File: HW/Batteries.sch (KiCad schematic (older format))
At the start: 18 parts

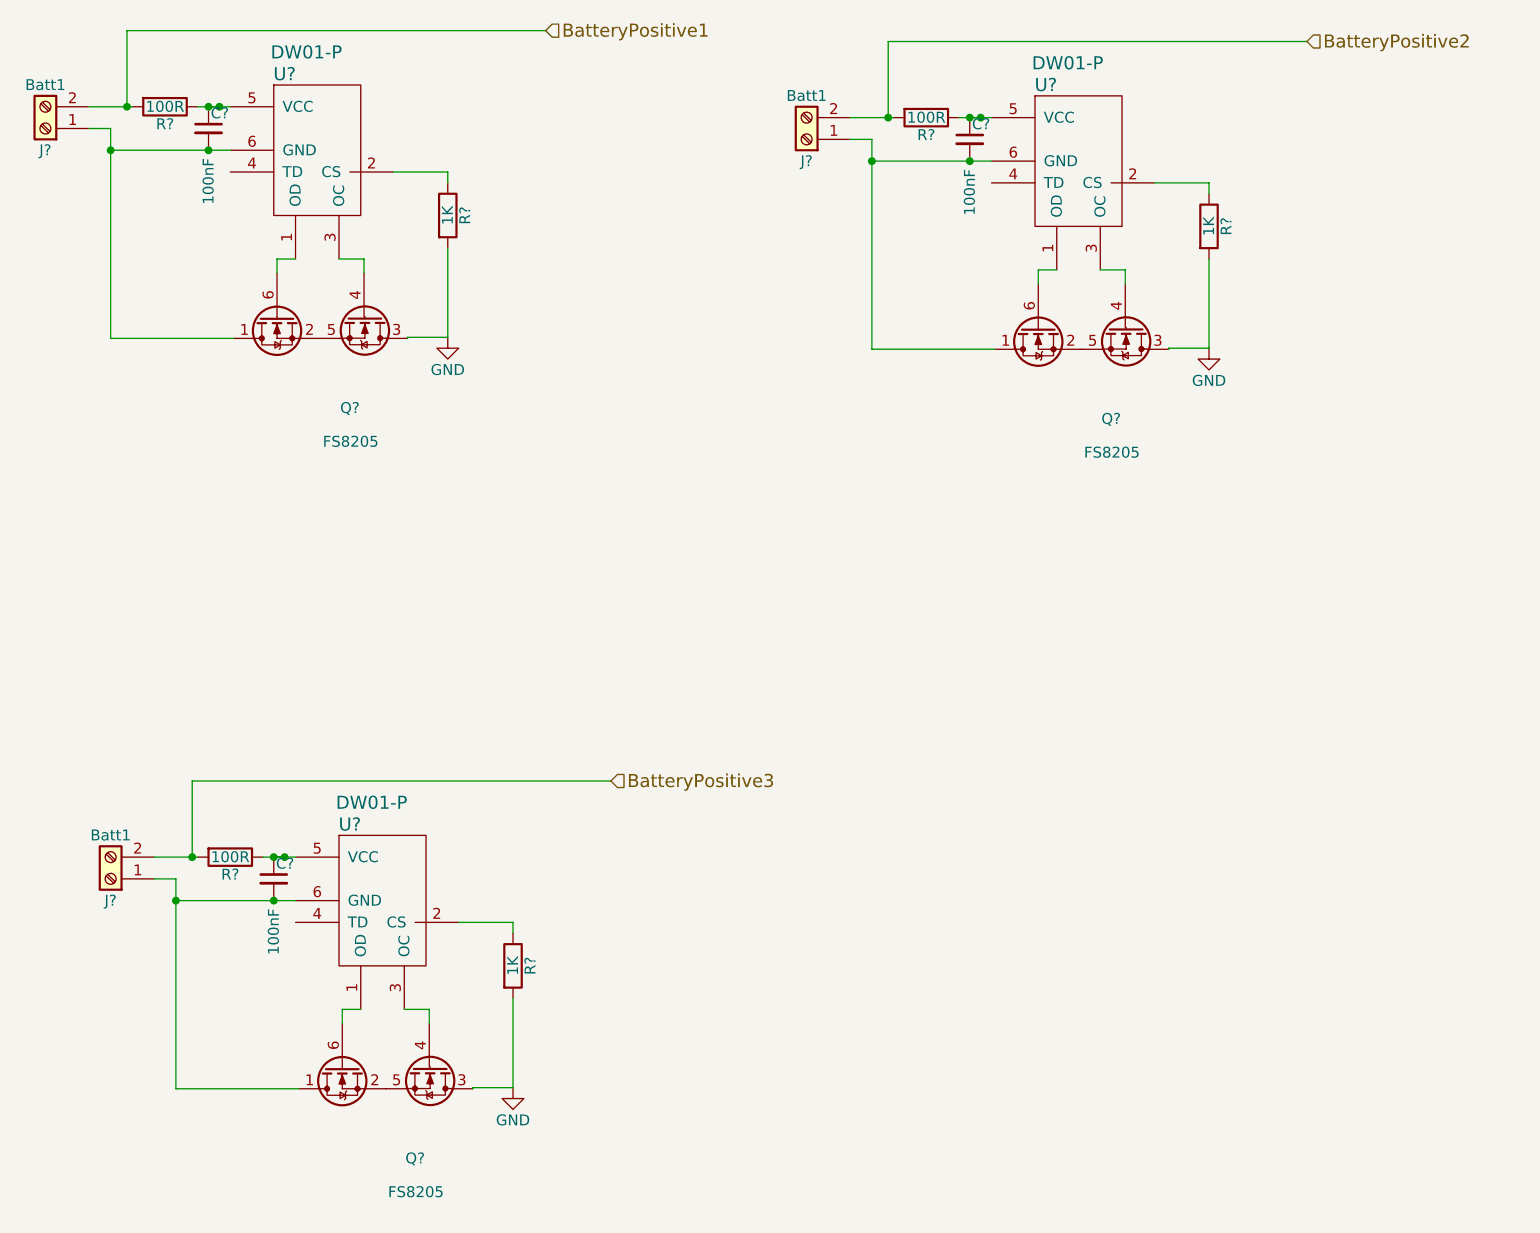
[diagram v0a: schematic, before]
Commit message: Add files via upload
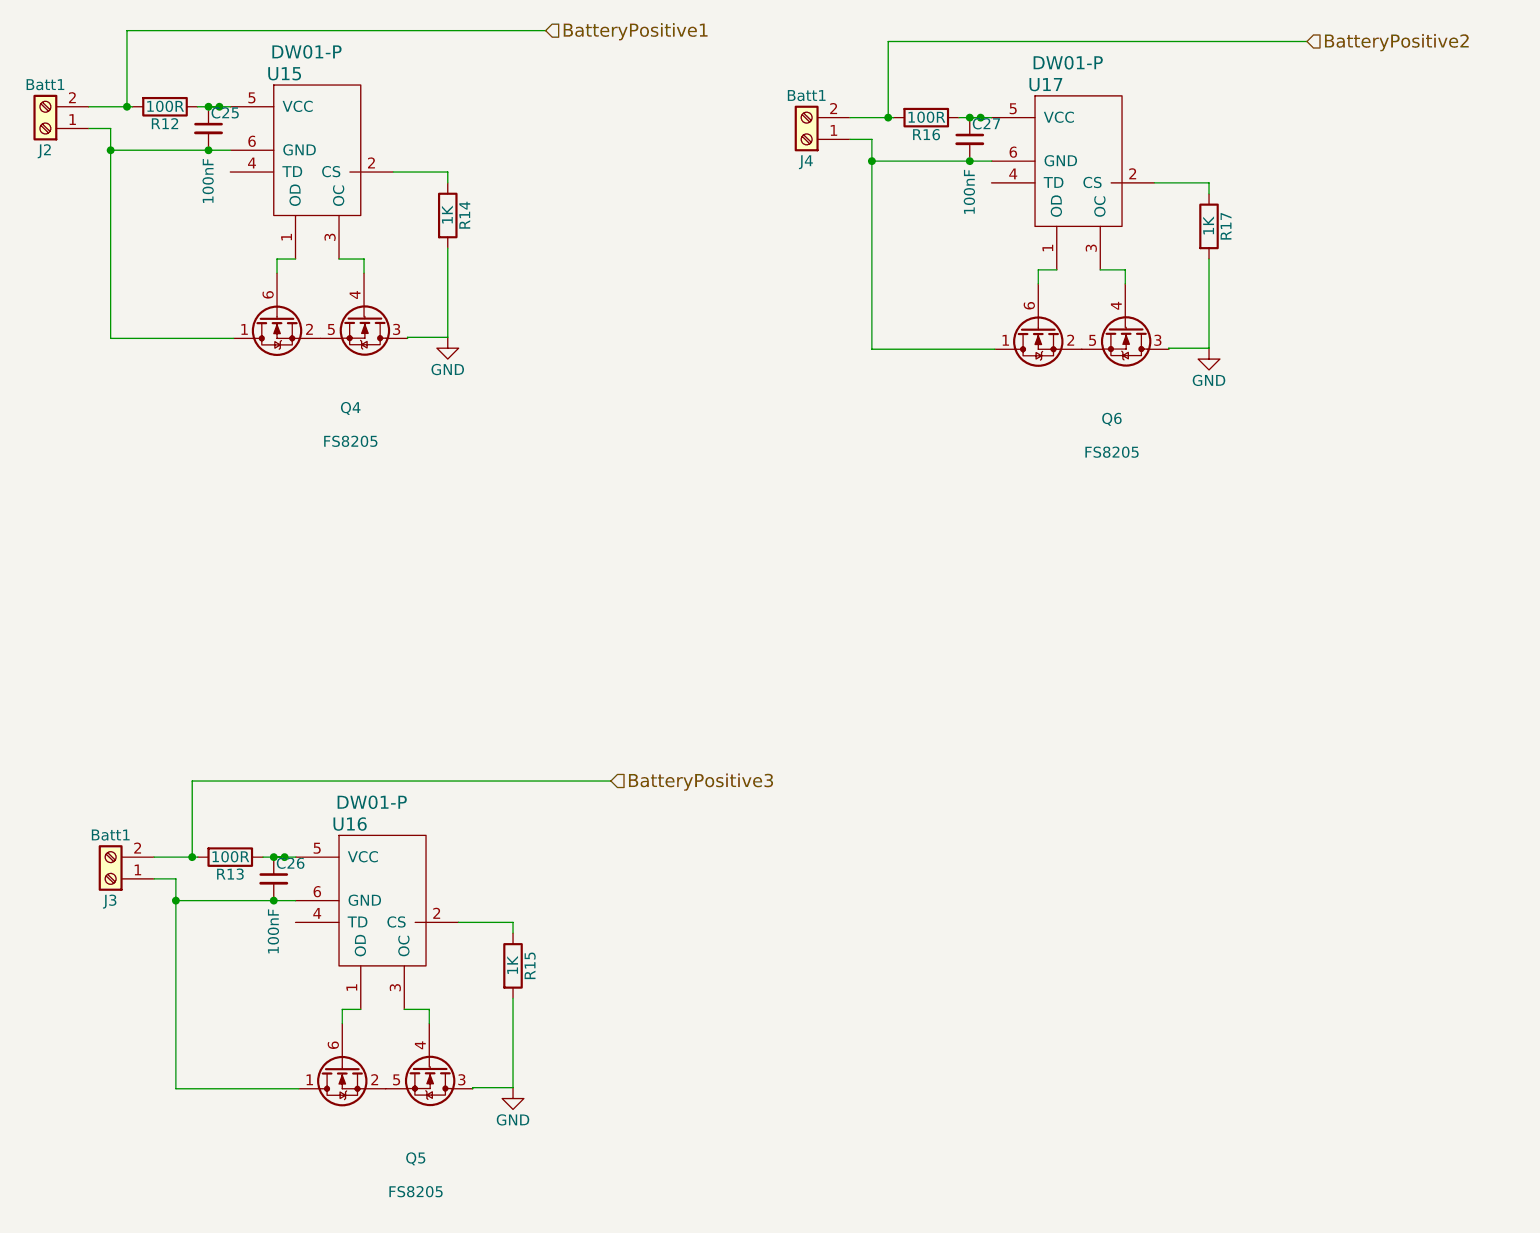
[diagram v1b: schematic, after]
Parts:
- C25, C26, C27: renamed from C?; footprint (none) -> Capacitors_SMD:C_0805_HandSoldering
- J2, J3, J4: renamed from J?; footprint (none) -> Connectors_Terminal_Blocks:TerminalBlock_bornier-2_P5.08mm
- R12, R13, R14, R15, R16, R17: renamed from R?; footprint (none) -> Resistors_SMD:R_0805_HandSoldering
- gave numbers to parts that had none: 6
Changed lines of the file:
@@
 LIBS:Peters
 LIBS:WS2812B
-LIBS:pro-mini-cache
+LIBS:discharger-cache
 EELAYER 25 0
 EELAYER END
@@
 BatteryPositive3
 $Comp
-L R R?
+L R R16
 U 1 1 5A983102
 P 5350 1600
-F 0 "R?" V 5430 1600 50  0000 C CNN
+F 0 "R16" V 5430 1600 50  0000 C CNN
 F 1 "100R" V 5350 1600 50  0000 C CNN
-F 2 "" V 5280 1600 50  0001 C CNN
+F 2 "Resistors_SMD:R_0805_HandSoldering" V 5280 1600 50  0001 C CNN
 F 3 "" H 5350 1600 50  0001 C CNN
 	1    5350 1600
@@
 $EndComp
 $Comp
-L C_Small C?
+L C_Small C27
 U 1 1 5A983108
 P 5550 1700
-F 0 "C?" H 5560 1770 50  0000 L CNN
+F 0 "C27" H 5560 1770 50  0000 L CNN
 F 1 "100nF" V 5550 1350 50  0000 L CNN
-F 2 "" H 5550 1700 50  0001 C CNN
+F 2 "Capacitors_SMD:C_0805_HandSoldering" H 5550 1700 50  0001 C CNN
 F 3 "" H 5550 1700 50  0001 C CNN
 	1    5550 1700
@@
 $EndComp
 $Comp
-L R R?
+L R R17
 U 1 1 5A98310E
 P 6650 2100
-F 0 "R?" V 6730 2100 50  0000 C CNN
+F 0 "R17" V 6730 2100 50  0000 C CNN
 F 1 "1K" V 6650 2100 50  0000 C CNN
-F 2 "" V 6580 2100 50  0001 C CNN
+F 2 "Resistors_SMD:R_0805_HandSoldering" V 6580 2100 50  0001 C CNN
 F 3 "" H 6650 2100 50  0001 C CNN
 	1    6650 2100
@@
 $EndComp
 $Comp
-L FS8205 Q?
+L FS8205 Q6
 U 1 1 5A983114
 P 6065 2665
-F 0 "Q?" H 6155 2345 50  0000 L CNN
+F 0 "Q6" H 6155 2345 50  0000 L CNN
 F 1 "FS8205" H 6075 2190 50  0000 L CNN
 F 2 "TO_SOT_Packages_SMD:SOT-23-6_Handsoldering" H 5125 2065 50  0001 L CIN
@@
 $EndComp
 $Comp
-L Screw_Terminal_01x02 J?
+L Screw_Terminal_01x02 J4
 U 1 1 5A98311A
 P 4800 1700
-F 0 "J?" H 4800 1800 50  0000 C CNN
+F 0 "J4" H 4800 1800 50  0000 C CNN
 F 1 "Batt1" H 4800 1500 50  0000 C CNN
-F 2 "" H 4800 1700 50  0001 C CNN
+F 2 "Connectors_Terminal_Blocks:TerminalBlock_bornier-2_P5.08mm" H 4800 1700 50  0001 C CNN
 F 3 "" H 4800 1700 50  0001 C CNN
 	1    4800 1700
@@
 $EndComp
 $Comp
-L GND #PWR?
+L GND #PWR92
 U 1 1 5A983120
 P 6650 2660
-F 0 "#PWR?" H 6650 2410 50  0001 C CNN
+F 0 "#PWR92" H 6650 2410 50  0001 C CNN
 F 1 "GND" H 6650 2510 50  0000 C CNN
 F 2 "" H 6650 2660 50  0001 C CNN
@@
 Connection ~ 5175 1600
 $Comp
-L DW01-P U?
+L DW01-P U17
 U 1 1 5A983132
 P 6000 1700
-F 0 "U?" H 5900 1950 60  0000 C CNN
+F 0 "U17" H 5900 1950 60  0000 C CNN
 F 1 "DW01-P" H 6000 2050 60  0000 C CNN
 F 2 "TO_SOT_Packages_SMD:SOT-23-6_Handsoldering" H 5750 2150 60  0001 C CNN
@@
 	5100 1800 5650 1800
 $Comp
-L R R?
+L R R12
 U 1 1 5A983DEE
 P 1850 1550
-F 0 "R?" V 1930 1550 50  0000 C CNN
+F 0 "R12" V 1930 1550 50  0000 C CNN
 F 1 "100R" V 1850 1550 50  0000 C CNN
-F 2 "" V 1780 1550 50  0001 C CNN
+F 2 "Resistors_SMD:R_0805_HandSoldering" V 1780 1550 50  0001 C CNN
 F 3 "" H 1850 1550 50  0001 C CNN
 	1    1850 1550
@@
 $EndComp
 $Comp
-L C_Small C?
+L C_Small C25
 U 1 1 5A983DF4
 P 2050 1650
-F 0 "C?" H 2060 1720 50  0000 L CNN
+F 0 "C25" H 2060 1720 50  0000 L CNN
 F 1 "100nF" V 2050 1300 50  0000 L CNN
-F 2 "" H 2050 1650 50  0001 C CNN
+F 2 "Capacitors_SMD:C_0805_HandSoldering" H 2050 1650 50  0001 C CNN
 F 3 "" H 2050 1650 50  0001 C CNN
 	1    2050 1650
@@
 $EndComp
 $Comp
-L R R?
+L R R14
 U 1 1 5A983DFA
 P 3150 2050
-F 0 "R?" V 3230 2050 50  0000 C CNN
+F 0 "R14" V 3230 2050 50  0000 C CNN
 F 1 "1K" V 3150 2050 50  0000 C CNN
-F 2 "" V 3080 2050 50  0001 C CNN
+F 2 "Resistors_SMD:R_0805_HandSoldering" V 3080 2050 50  0001 C CNN
 F 3 "" H 3150 2050 50  0001 C CNN
 	1    3150 2050
@@
 $EndComp
 $Comp
-L FS8205 Q?
+L FS8205 Q4
 U 1 1 5A983E00
 P 2565 2615
-F 0 "Q?" H 2655 2295 50  0000 L CNN
+F 0 "Q4" H 2655 2295 50  0000 L CNN
 F 1 "FS8205" H 2575 2140 50  0000 L CNN
 F 2 "TO_SOT_Packages_SMD:SOT-23-6_Handsoldering" H 1625 2015 50  0001 L CIN
@@
 $EndComp
 $Comp
-L Screw_Terminal_01x02 J?
+L Screw_Terminal_01x02 J2
 U 1 1 5A983E06
 P 1300 1650
-F 0 "J?" H 1300 1750 50  0000 C CNN
+F 0 "J2" H 1300 1750 50  0000 C CNN
 F 1 "Batt1" H 1300 1450 50  0000 C CNN
-F 2 "" H 1300 1650 50  0001 C CNN
+F 2 "Connectors_Terminal_Blocks:TerminalBlock_bornier-2_P5.08mm" H 1300 1650 50  0001 C CNN
 F 3 "" H 1300 1650 50  0001 C CNN
 	1    1300 1650
@@
 $EndComp
 $Comp
-L GND #PWR?
+L GND #PWR90
 U 1 1 5A983E0C
 P 3150 2610
-F 0 "#PWR?" H 3150 2360 50  0001 C CNN
+F 0 "#PWR90" H 3150 2360 50  0001 C CNN
 F 1 "GND" H 3150 2460 50  0000 C CNN
 F 2 "" H 3150 2610 50  0001 C CNN
@@
 Connection ~ 1675 1550
 $Comp
-L DW01-P U?
+L DW01-P U15
 U 1 1 5A983E19
 P 2500 1650
-F 0 "U?" H 2400 1900 60  0000 C CNN
+F 0 "U15" H 2400 1900 60  0000 C CNN
 F 1 "DW01-P" H 2500 2000 60  0000 C CNN
 F 2 "TO_SOT_Packages_SMD:SOT-23-6_Handsoldering" H 2250 2100 60  0001 C CNN
@@
 	1600 1750 2150 1750
 $Comp
-L R R?
+L R R13
 U 1 1 5A984135
 P 2150 5000
-F 0 "R?" V 2230 5000 50  0000 C CNN
+F 0 "R13" V 2230 5000 50  0000 C CNN
 F 1 "100R" V 2150 5000 50  0000 C CNN
-F 2 "" V 2080 5000 50  0001 C CNN
+F 2 "Resistors_SMD:R_0805_HandSoldering" V 2080 5000 50  0001 C CNN
 F 3 "" H 2150 5000 50  0001 C CNN
 	1    2150 5000
@@
 $EndComp
 $Comp
-L C_Small C?
+L C_Small C26
 U 1 1 5A98413B
 P 2350 5100
-F 0 "C?" H 2360 5170 50  0000 L CNN
+F 0 "C26" H 2360 5170 50  0000 L CNN
 F 1 "100nF" V 2350 4750 50  0000 L CNN
-F 2 "" H 2350 5100 50  0001 C CNN
+F 2 "Capacitors_SMD:C_0805_HandSoldering" H 2350 5100 50  0001 C CNN
 F 3 "" H 2350 5100 50  0001 C CNN
 	1    2350 5100
@@
 $EndComp
 $Comp
-L R R?
+L R R15
 U 1 1 5A984141
 P 3450 5500
-F 0 "R?" V 3530 5500 50  0000 C CNN
+F 0 "R15" V 3530 5500 50  0000 C CNN
 F 1 "1K" V 3450 5500 50  0000 C CNN
-F 2 "" V 3380 5500 50  0001 C CNN
+F 2 "Resistors_SMD:R_0805_HandSoldering" V 3380 5500 50  0001 C CNN
 F 3 "" H 3450 5500 50  0001 C CNN
 	1    3450 5500
@@
 $EndComp
 $Comp
-L FS8205 Q?
+L FS8205 Q5
 U 1 1 5A984147
 P 2865 6065
-F 0 "Q?" H 2955 5745 50  0000 L CNN
+F 0 "Q5" H 2955 5745 50  0000 L CNN
 F 1 "FS8205" H 2875 5590 50  0000 L CNN
 F 2 "TO_SOT_Packages_SMD:SOT-23-6_Handsoldering" H 1925 5465 50  0001 L CIN
@@
 $EndComp
 $Comp
-L Screw_Terminal_01x02 J?
+L Screw_Terminal_01x02 J3
 U 1 1 5A98414D
 P 1600 5100
-F 0 "J?" H 1600 5200 50  0000 C CNN
+F 0 "J3" H 1600 5200 50  0000 C CNN
 F 1 "Batt1" H 1600 4900 50  0000 C CNN
-F 2 "" H 1600 5100 50  0001 C CNN
+F 2 "Connectors_Terminal_Blocks:TerminalBlock_bornier-2_P5.08mm" H 1600 5100 50  0001 C CNN
 F 3 "" H 1600 5100 50  0001 C CNN
 	1    1600 5100
@@
 $EndComp
 $Comp
-L GND #PWR?
+L GND #PWR91
 U 1 1 5A984153
 P 3450 6060
-F 0 "#PWR?" H 3450 5810 50  0001 C CNN
+F 0 "#PWR91" H 3450 5810 50  0001 C CNN
 F 1 "GND" H 3450 5910 50  0000 C CNN
 F 2 "" H 3450 6060 50  0001 C CNN
@@
 Connection ~ 1975 5000
 $Comp
-L DW01-P U?
+L DW01-P U16
 U 1 1 5A984160
 P 2800 5100
-F 0 "U?" H 2700 5350 60  0000 C CNN
+F 0 "U16" H 2700 5350 60  0000 C CNN
 F 1 "DW01-P" H 2800 5450 60  0000 C CNN
 F 2 "TO_SOT_Packages_SMD:SOT-23-6_Handsoldering" H 2550 5550 60  0001 C CNN
